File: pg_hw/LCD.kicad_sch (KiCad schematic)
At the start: 1 part, among them J4 ILI1934

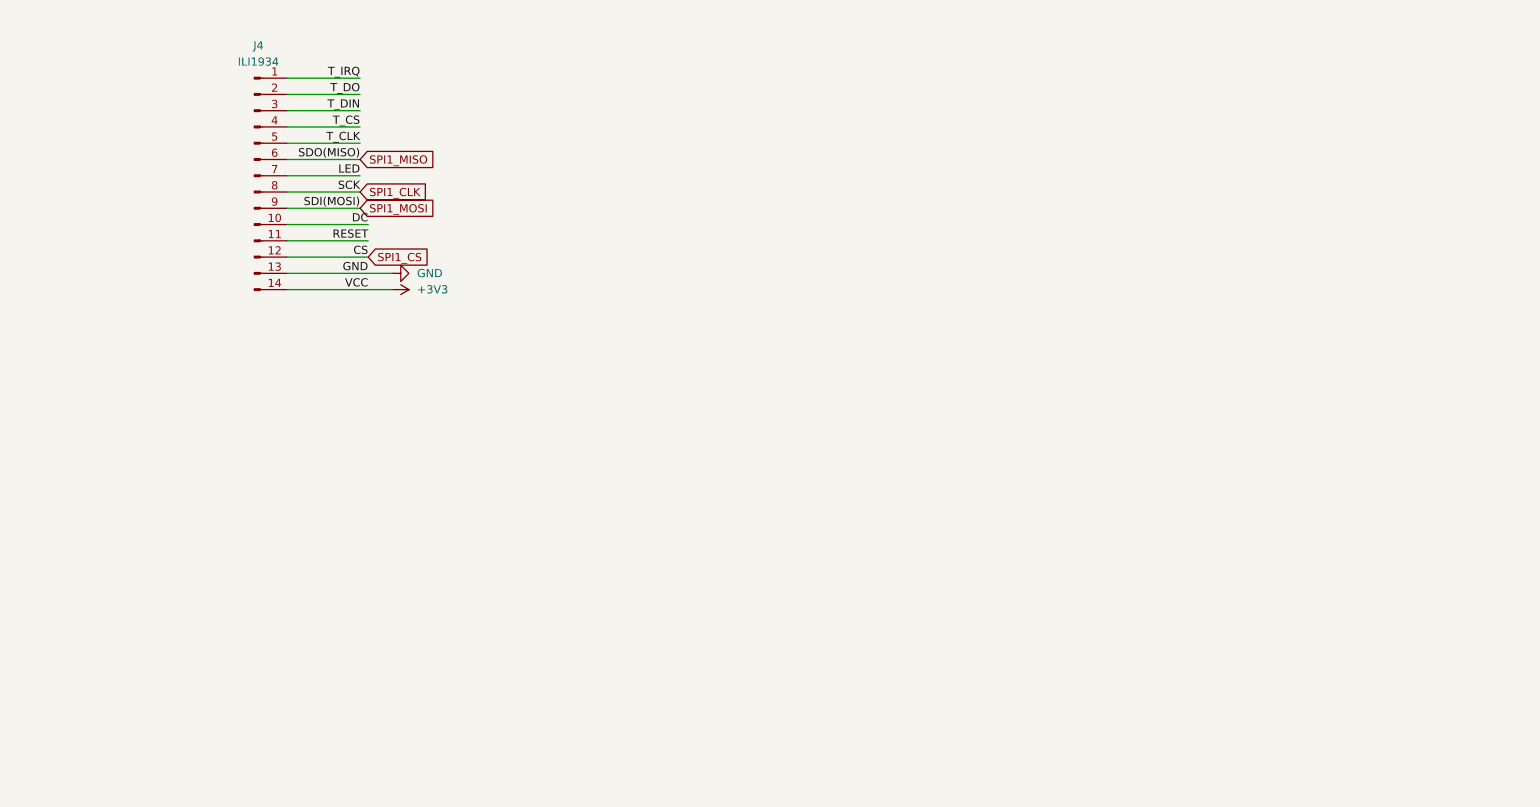
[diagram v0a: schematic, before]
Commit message: push
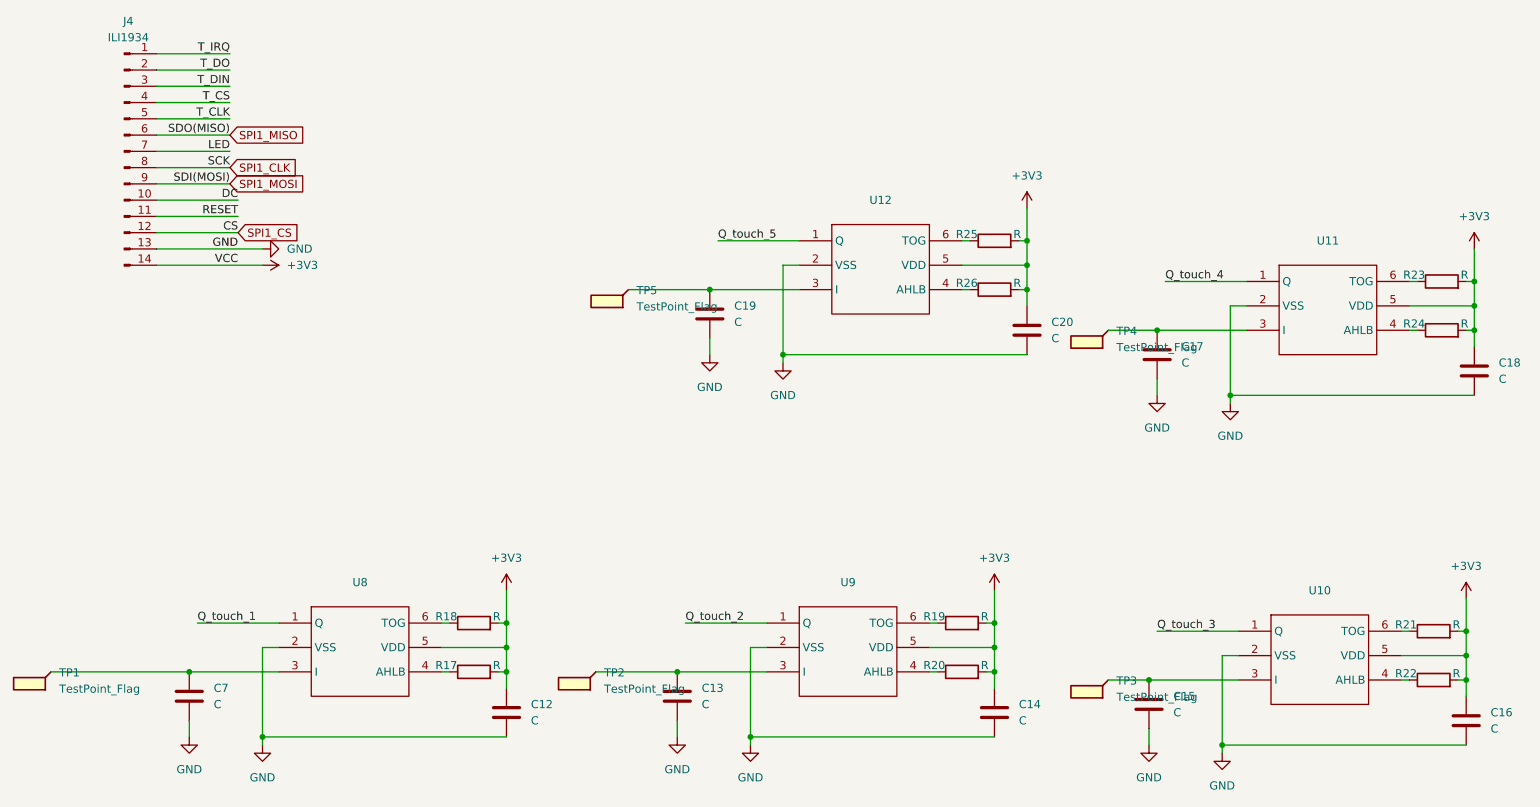
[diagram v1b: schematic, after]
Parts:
- added C12, C13, C14, C15, C16, C17, C18, C19, C20, C7: C, symbol Device:C
- added R17, R18, R19, R20, R21, R22, R23, R24, R25, R26: R, symbol Device:R
- added TP1, TP2, TP3, TP4, TP5: TestPoint_Flag, symbol Connector:TestPoint_Flag
- added U10, U11, U12, U8, U9: ~, symbol TTP:ttp233
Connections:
- net +3V3: now also C12.1, C14.1, C16.1, C18.1, C20.1, R17.2, R18.2, R19.2, R20.2, R21.2, R22.2, R23.2, R24.2, R25.2, R26.2, U10.5 (VDD), U11.5 (VDD), U12.5 (VDD), U8.5 (VDD), U9.5 (VDD)
- net GND: now also C12.2, C13.2, C14.2, C15.2, C16.2, C17.2, C18.2, C19.2, C20.2, C7.2, U10.2 (VSS), U11.2 (VSS), U12.2 (VSS), U8.2 (VSS), U9.2 (VSS)
- new net: R18.1, U8.6 (TOG)
- new net: C15.1, TP3.1, U10.3 (I)
- new net: R22.1, U10.4 (AHLB)
- new net: R21.1, U10.6 (TOG)
- new net: C13.1, TP2.1, U9.3 (I)
- new net: R20.1, U9.4 (AHLB)
- new net: R19.1, U9.6 (TOG)
- new net: C7.1, TP1.1, U8.3 (I)
- new net: R17.1, U8.4 (AHLB)
- new net: R23.1, U11.6 (TOG)
- new net: C19.1, TP5.1, U12.3 (I)
- new net: C17.1, TP4.1, U11.3 (I)
- new net: R24.1, U11.4 (AHLB)
- new net: R25.1, U12.6 (TOG)
- new net: R26.1, U12.4 (AHLB)
- new net Q_touch_1: U8.1 (Q)
- new net Q_touch_2: U9.1 (Q)
- new net Q_touch_3: U10.1 (Q)
- new net Q_touch_4: U11.1 (Q)
- new net Q_touch_5: U12.1 (Q)
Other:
- moved on the sheet: J4
